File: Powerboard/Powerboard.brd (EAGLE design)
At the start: 87.5 x 150 mm, 10 parts

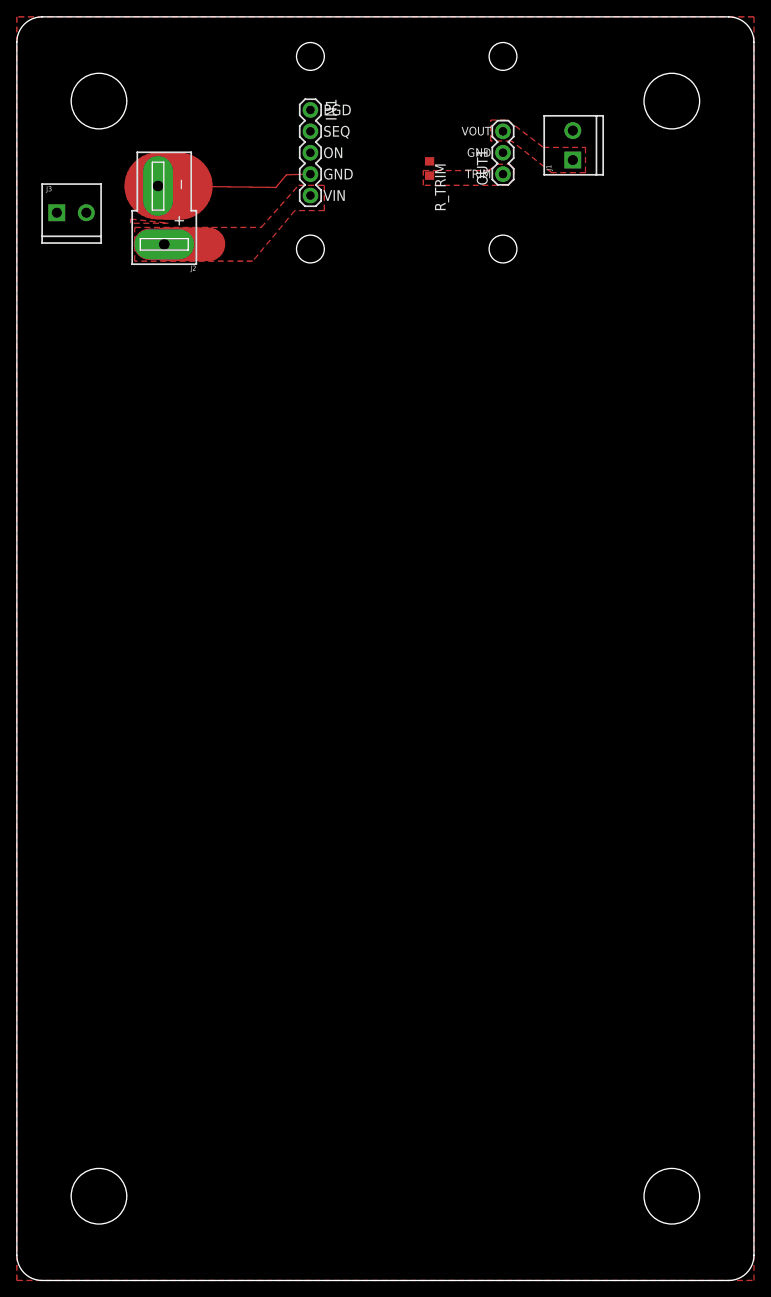
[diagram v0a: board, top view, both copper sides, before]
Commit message: wip
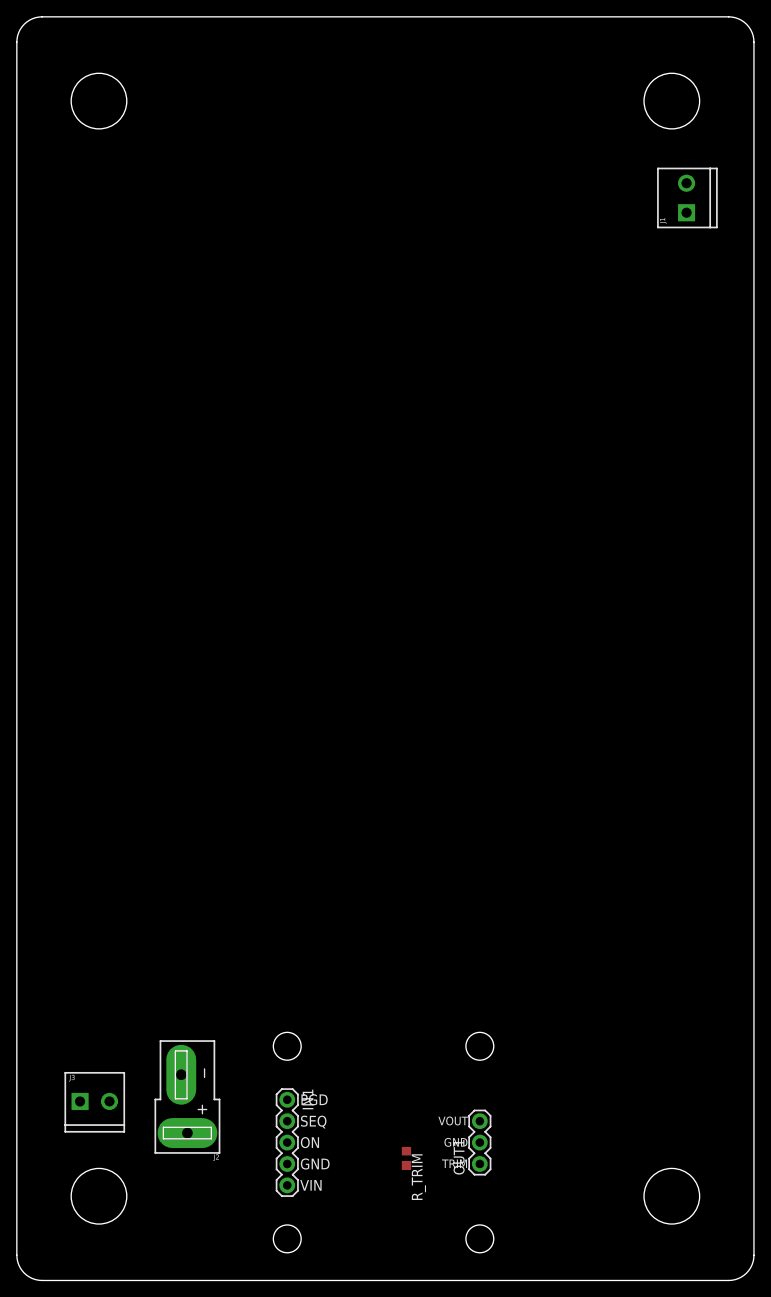
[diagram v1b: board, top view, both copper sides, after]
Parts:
- moved OUT1 117.5 mm to (55.0, 13.8)
- moved U$2 117.5 mm to (32.1, 27.8)
- moved U$7 117.5 mm to (55.0, 27.8)
- moved R_TRIM 117.5 mm to (46.2, 14.5)
- moved U$6 117.5 mm to (32.1, 4.94)
- moved U$8 117.5 mm to (55.0, 4.94)
- moved IN1 117.5 mm to (32.1, 21.4)
- moved J2 105.5 mm to (20.2, 17.5)
- moved J3 105.5 mm to (7.50, 21.2)
- moved J1 14.9 mm to (79.5, 126.8)
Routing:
- net GND: track 18.8 -> 0.00 mm
- net VIN: track 7.50 -> 0.00 mm
- removed copper zone on layer 1, net GND
- removed copper zone on layer 1, net TRIM
- removed copper zone on layer 1, net VIN
- removed copper zone on layer 1, net VOUT
